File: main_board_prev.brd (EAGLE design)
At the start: 119 x 65 mm, 49 parts, among them IC1 LT1168ACS8, IC2 LT1168ACS8, IC3 LT1168ACS8, IC4 317EMP, U1 TLC272IP, U2 TLC272IP, U3 TLC272IP

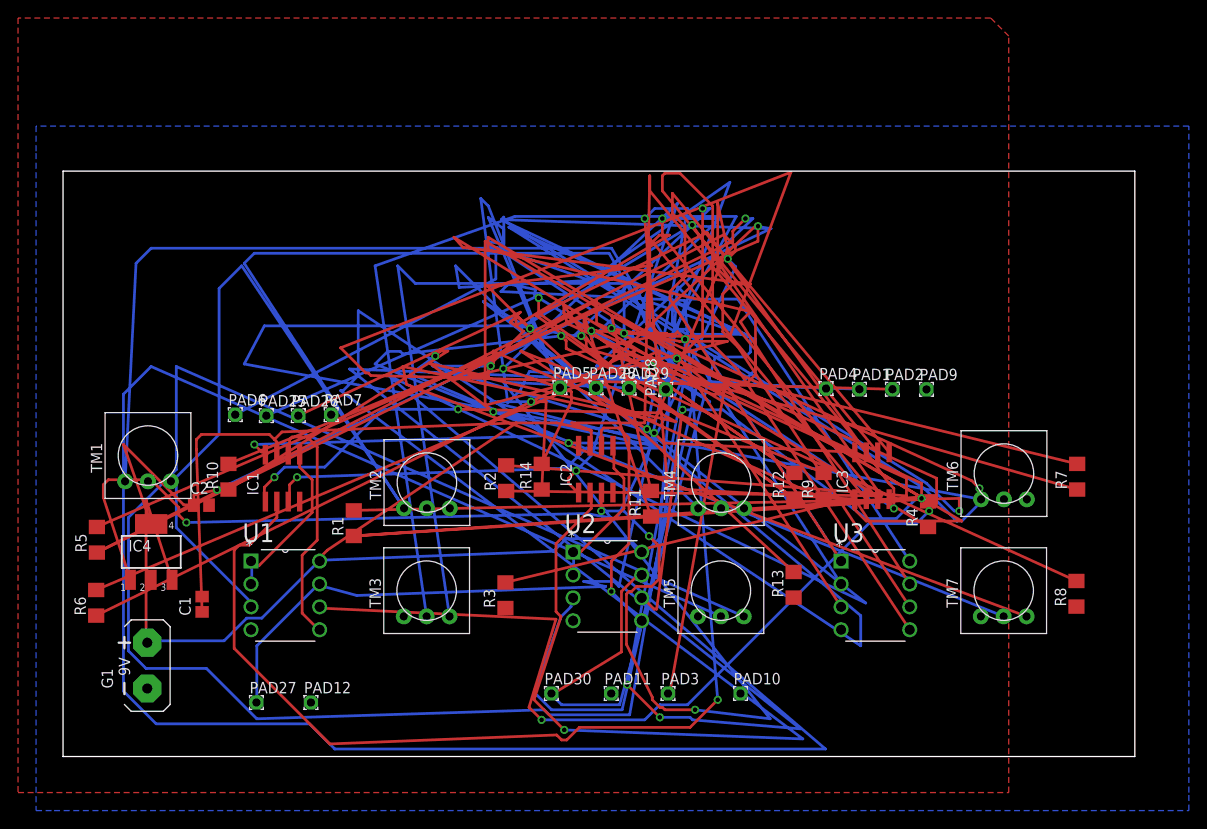
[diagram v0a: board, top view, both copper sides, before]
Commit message: Re-doing main board. Use this
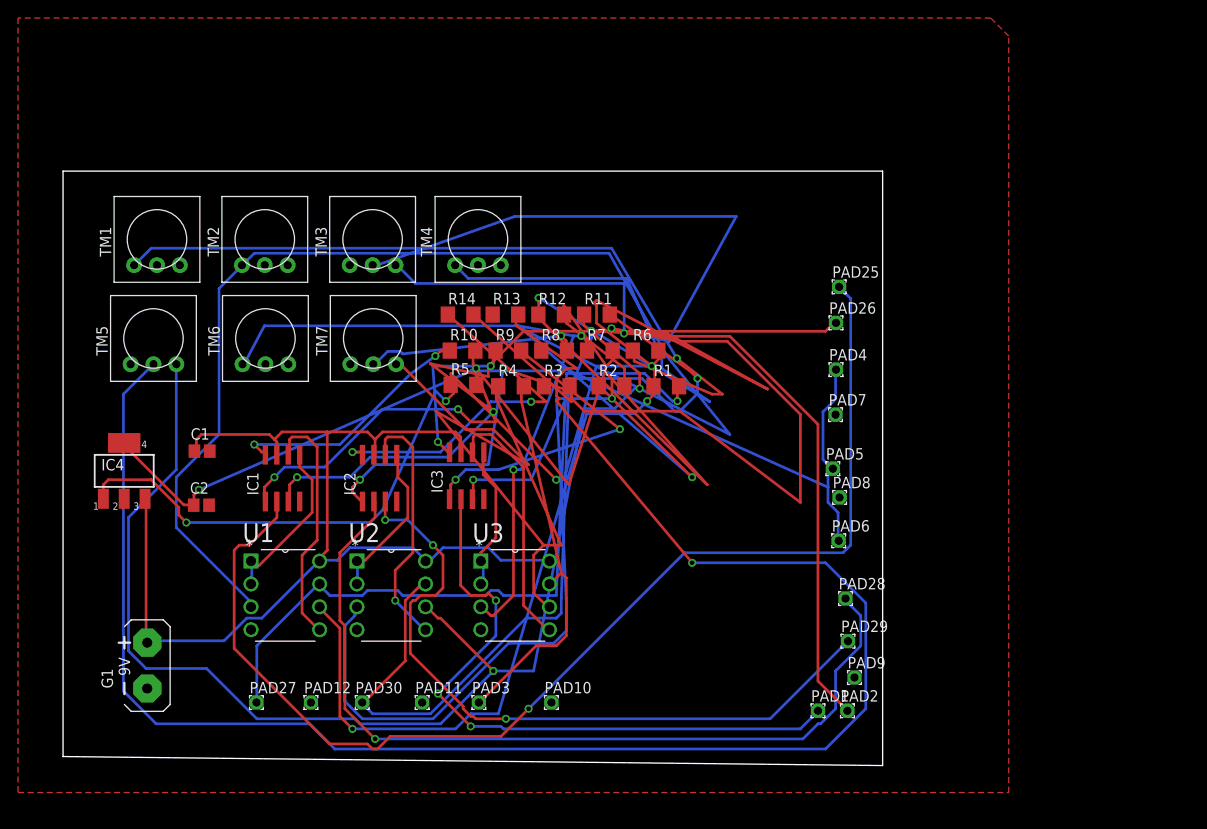
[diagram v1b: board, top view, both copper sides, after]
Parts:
- moved TM6 83.4 mm to (22.5, 46.4)
- moved TM7 75.4 mm to (34.4, 46.4)
- moved TM5 68.9 mm to (10.0, 46.4)
- moved PAD6 68.4 mm to (86.1, 24.0)
- moved R6 67.1 mm to (64.7, 45.1), turned to 0 degrees
- moved PAD25 65.2 mm to (86.2, 52.1)
- moved R8 64.0 mm to (54.5, 45.1), turned to 0 degrees
- moved PAD26 60.6 mm to (85.8, 48.1)
- moved PAD7 56.0 mm to (85.8, 38.0)
- moved R7 54.8 mm to (59.6, 45.1), turned to 0 degrees
- moved R4 48.4 mm to (49.7, 41.1), turned to 0 degrees
- moved IC3 45.0 mm to (44.8, 31.2)
- moved R5 44.2 mm to (44.5, 41.3), turned to 0 degrees
- moved R13 43.9 mm to (49.1, 49.1), turned to 0 degrees
- moved U3 40.0 mm to (54.0, 14.1)
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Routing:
- net VDD: track 593.6 -> 164.7 mm
- net N$6: track 367.1 -> 94.3 mm
- net N$27: track 462.7 -> 196.0 mm
- net N$2: track 387.2 -> 159.7 mm
- net VCC: track 330.0 -> 120.0 mm
- net N$25: track 382.3 -> 180.2 mm
- net N$8: track 279.7 -> 79.9 mm
- net N$11: track 256.2 -> 77.8 mm
- net N$24: track 319.7 -> 143.0 mm
- net N$1: track 249.6 -> 83.9 mm
- net N$32: track 260.9 -> 96.3 mm
- net N$18: track 232.5 -> 72.1 mm
- net N$5: track 276.6 -> 128.8 mm
- net N$9: track 156.5 -> 16.2 mm
- net N$13: track 160.6 -> 23.6 mm
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- removed copper zone on layer 16, net N$33
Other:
- board size 119 x 65 mm -> 91 x 66 mm
